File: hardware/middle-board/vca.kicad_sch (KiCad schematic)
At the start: 22 parts, among them Q1 2N3904, Q2 2N3906, U1 TL084, U4 NE5517

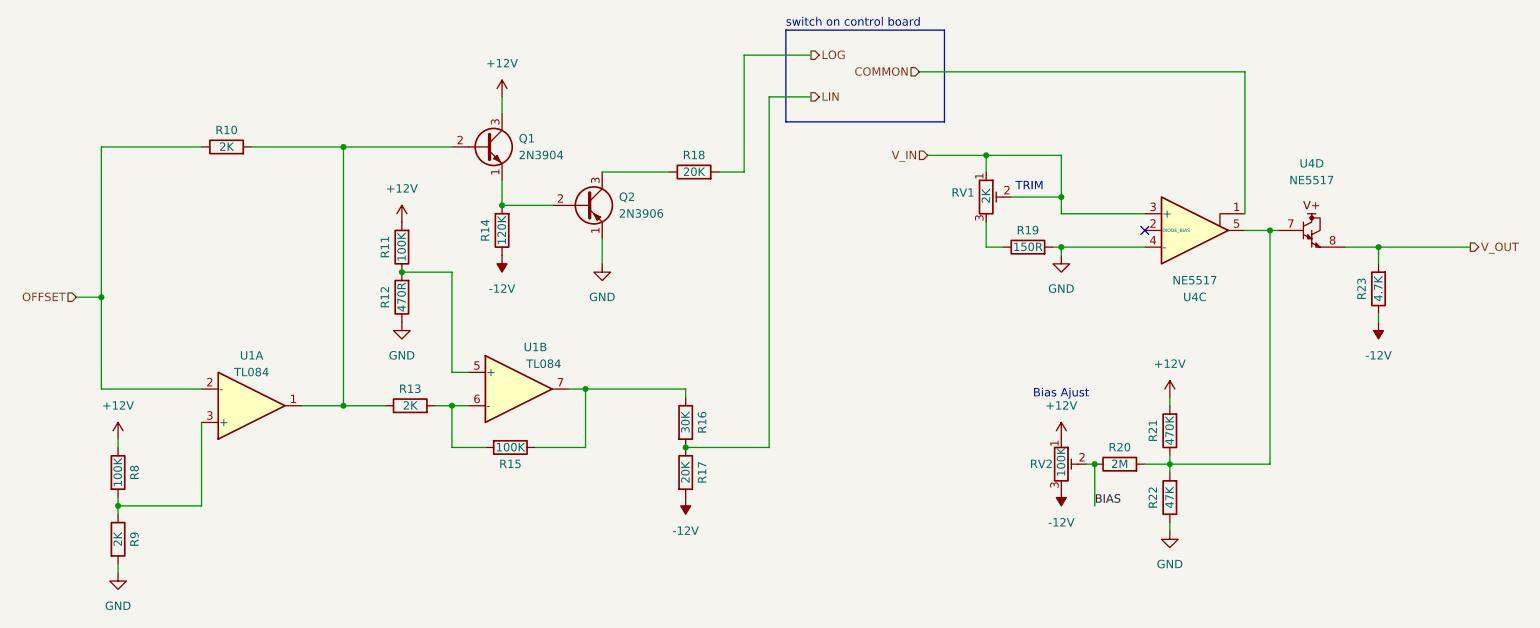
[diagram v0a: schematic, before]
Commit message: wip - first pass done
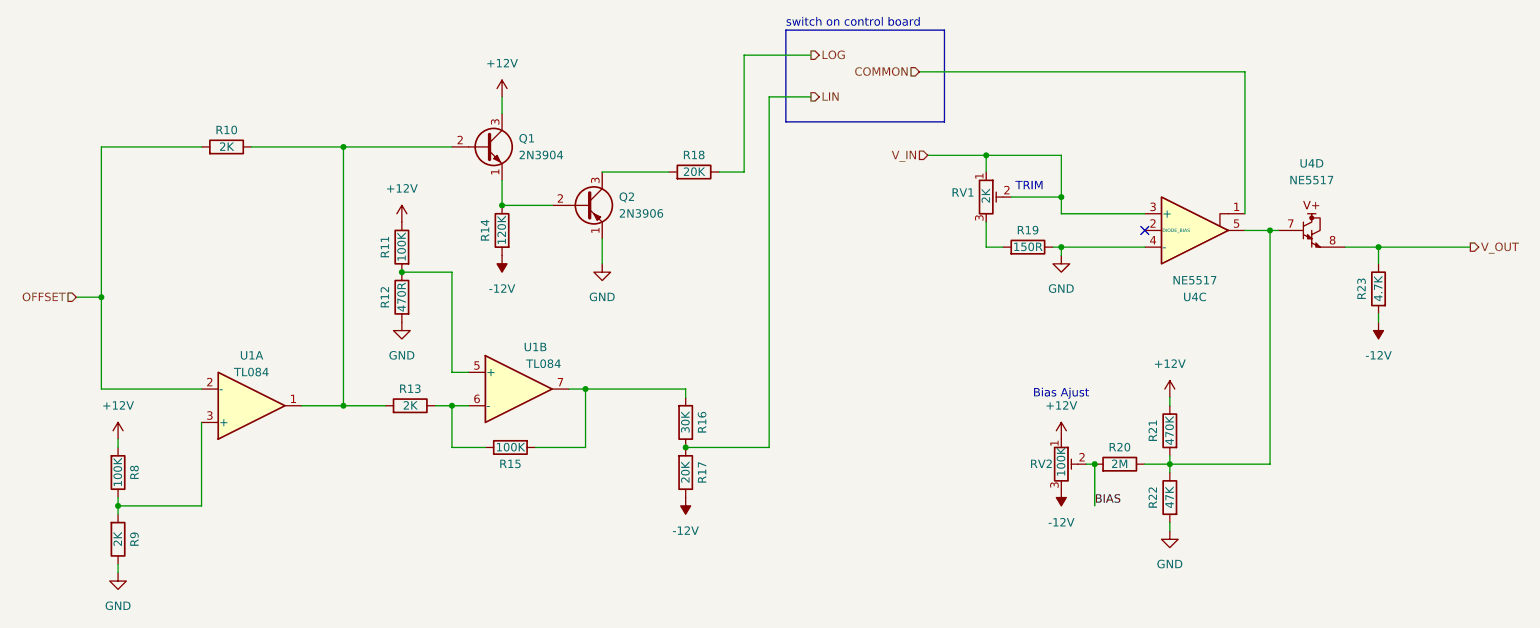
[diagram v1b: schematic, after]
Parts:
- Q1: footprint Package_TO_SOT_THT:TO-92_Inline -> Eurorack Common:TO-92_Inline; symbol Transistor_BJT:2N3904 -> Eurorack Common:2N3904
- Q2: footprint Package_TO_SOT_THT:TO-92_Inline -> Eurorack Common:TO-92_Inline; symbol Transistor_BJT:2N3906 -> Eurorack Common:2N3906
- R10, R11, R12, R13, R14, R15, R16, R17, R18, R19, R20, R21, R22, R23, R8, R9: footprint Resistor_THT:R_Axial_DIN0207_L6.3mm_D2.5mm_P7.62mm_Horizontal -> Eurorack Common:R_Axial_DIN0207_L6.3mm_D2.5mm_P7.62mm_Horizontal; symbol Device:R -> Eurorack Common:R_DIN0207
- U1: symbol Amplifier_Operational:TL084 -> Eurorack Common:TL084HIDYYR
- U4: footprint Package_SO:JEITA_SOIC-16_3.9x9.9mm_P1.27mm -> Eurorack Common:SOIC-16_3.9x9.9mm_P1.27mm; symbol Amplifier_Operational:LM13700 -> Eurorack Common:NE5517DR2G
